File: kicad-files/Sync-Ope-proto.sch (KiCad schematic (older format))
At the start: 59 parts, among them J1 rca, J10 rca, J2 euro_power, J3 mono_jack, J4 mono_jack, J5 mono_jack, J6 rca, J7 AC_POWER, J8 diy_power_header, J9 rca, U1 AD8072, U2 LM1881, U3 L7805, U4 L7905, U5 LT1251, U6 CD4053BE

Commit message: circuit revision 0.3
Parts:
- removed C14: 1nF, symbol Sync-Ope-proto-rescue:C-Device
- removed C3, C4: 100n, Capacitor_THT:C_Disc_D4.3mm_W1.9mm_P5.00mm, symbol Sync-Ope-proto-rescue:C-Sync-Ope-proto-Sync-Ope-proto-rescue
- removed CD4069: delay clamping signal, symbol Sync-Ope-proto-rescue:CD4069
- removed D1: video signal indicator LED, LED_THT:LED_D3.0mm, symbol Sync-Ope-proto-rescue:LED-Device
- removed D2, D3: 1n4148, Diode_THT:D_DO-35_SOD27_P7.62mm_Horizontal, symbol Sync-Ope-proto-rescue:D-Device
- removed R10: 100k, Resistor_THT:R_Axial_DIN0204_L3.6mm_D1.6mm_P7.62mm_Horizontal, symbol Sync-Ope-proto-rescue:R-Device
- removed R14: 10k, Resistor_THT:R_Axial_DIN0204_L3.6mm_D1.6mm_P7.62mm_Horizontal, symbol Sync-Ope-proto-rescue:R-Device
- removed R16: 39k, Resistor_THT:R_Axial_DIN0204_L3.6mm_D1.6mm_P7.62mm_Horizontal, symbol Sync-Ope-proto-rescue:R-Device
- removed R21: 3.3K, symbol Sync-Ope-proto-rescue:R-Device
- removed R3: 220, Resistor_THT:R_Axial_DIN0204_L3.6mm_D1.6mm_P7.62mm_Horizontal, symbol Sync-Ope-proto-rescue:R-Device
- removed R5: 1k, Resistor_THT:R_Axial_DIN0204_L3.6mm_D1.6mm_P7.62mm_Horizontal, symbol Sync-Ope-proto-rescue:R-Sync-Ope-proto-Sync-Ope-proto-rescue
- removed R9: 680k, Resistor_THT:R_Axial_DIN0204_L3.6mm_D1.6mm_P7.62mm_Horizontal, symbol Sync-Ope-proto-rescue:R-Sync-Ope-proto-Sync-Ope-proto-rescue
- removed U2: LM1881, Package_DIP:DIP-8_W7.62mm_LongPads, symbol Sync-Ope-proto-rescue:LM1881-Sync-Ope-proto-Sync-Ope-proto-rescue
- removed U6: CD4053BE, Package_DIP:DIP-16_W7.62mm_LongPads, symbol Sync-Ope-proto-rescue:4053-4xxx
- added C14, C15, C16, C17, C18, C19: 0.1u, Capacitor_THT:C_Disc_D4.3mm_W1.9mm_P5.00mm, symbol Device:C_Small
- added R3: 510, Resistor_THT:R_Axial_DIN0204_L3.6mm_D1.6mm_P7.62mm_Horizontal, symbol Sync-Ope-proto-rescue:R-Sync-Ope-proto-Sync-Ope-proto-rescue
- added R5: 39k, Resistor_THT:R_Axial_DIN0204_L3.6mm_D1.6mm_P7.62mm_Horizontal, symbol Sync-Ope-proto-rescue:R-Device
- C2, C5, C7, C9: value 100n -> 0.1u
- C6, C8: value 330n -> 0.33u
- D7: value schottky -> bat46
- J1, J10, J6, J9: footprint lib_fp:RCJ-024 -> lib_fp:tht_vertical_rca
- J2: value euro_power -> europower
- J3, J4, J5: value mono_jack -> mono_jack_3.5mm
- J7: value AC_POWER -> barrel_jack
- R18: symbol Sync-Ope-proto-rescue:R-Sync-Ope-proto-Sync-Ope-proto-rescue -> Device:R
- RV1: value 10k -> 10k_pot
- U1: footprint Package_DIP:DIP-8_W7.62mm_LongPads -> lib_fp:DIP-SOIC-8
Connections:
- net +5V: now also C14.1, C15.1, C16.1, C17.1, R5.1
- net -5V: now also C18.2, C19.2
- net GND: now also R12.1, C14.2, C15.2, C16.2, C17.2, C18.1, C19.1; no longer J4.TN, R12.2
- net at D6.1 (K), D7.1 (K), U5.1 (IN_1): now also R12.2, R13.1; no longer R12.1, R13.2
- net blanking/return_blank: now reaches J4.T, J9.1 (In)
- net blanking/return_blank: now also R13.2; no longer R13.1
- net at J5.TN: now also R5.2
- net blanking/control_blank: now reaches J5.T
- net ADDED_SYNC renamed blanking/control_pulse
- net DRY_BLANKED_SIGNAL renamed blanking/input_blank
- net VIDEO_TO_SYNC renamed blanking/video_in
- net blanking/video_in: now also R3.2; no longer U1.3 (+)
- new net: R3.1, U1.3 (+)
- no-connect marks 14 -> 12
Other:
- note added: "DRY/WET"
- note removed: "Signal Blanking"
- note removed: "Video Sync Seperator"
- moved on the sheet: C10, C11, C12, C13, C2, C5, C6, C7, C8, C9, D4, D5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

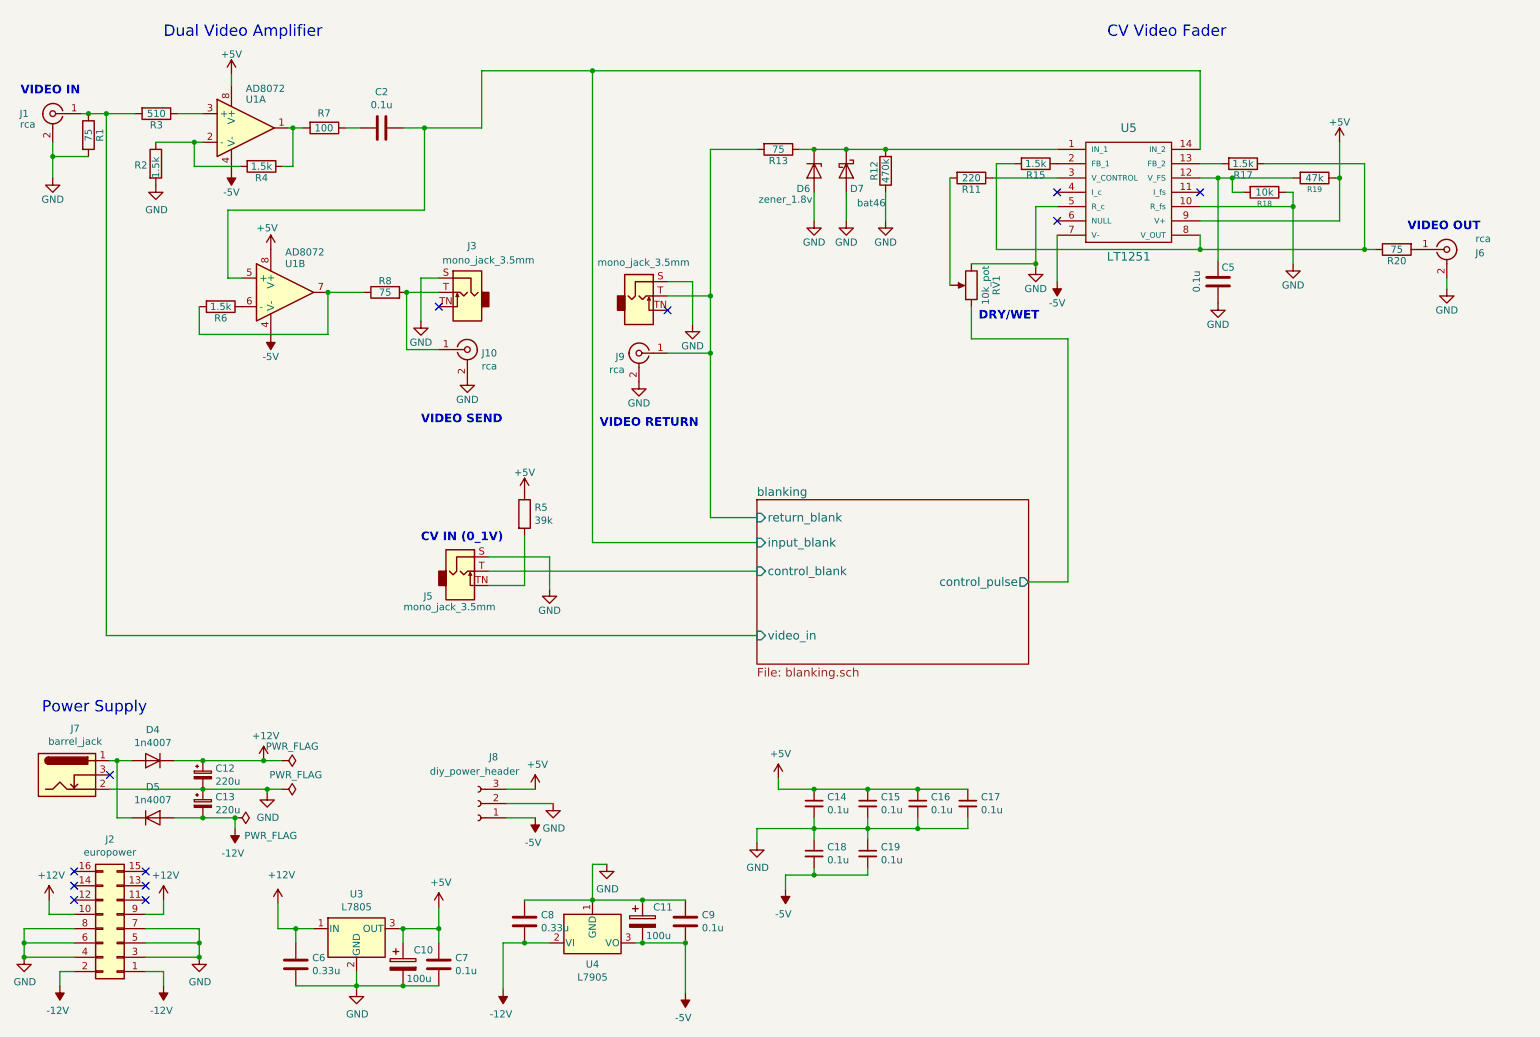
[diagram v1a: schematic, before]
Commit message: working on v0.4.0
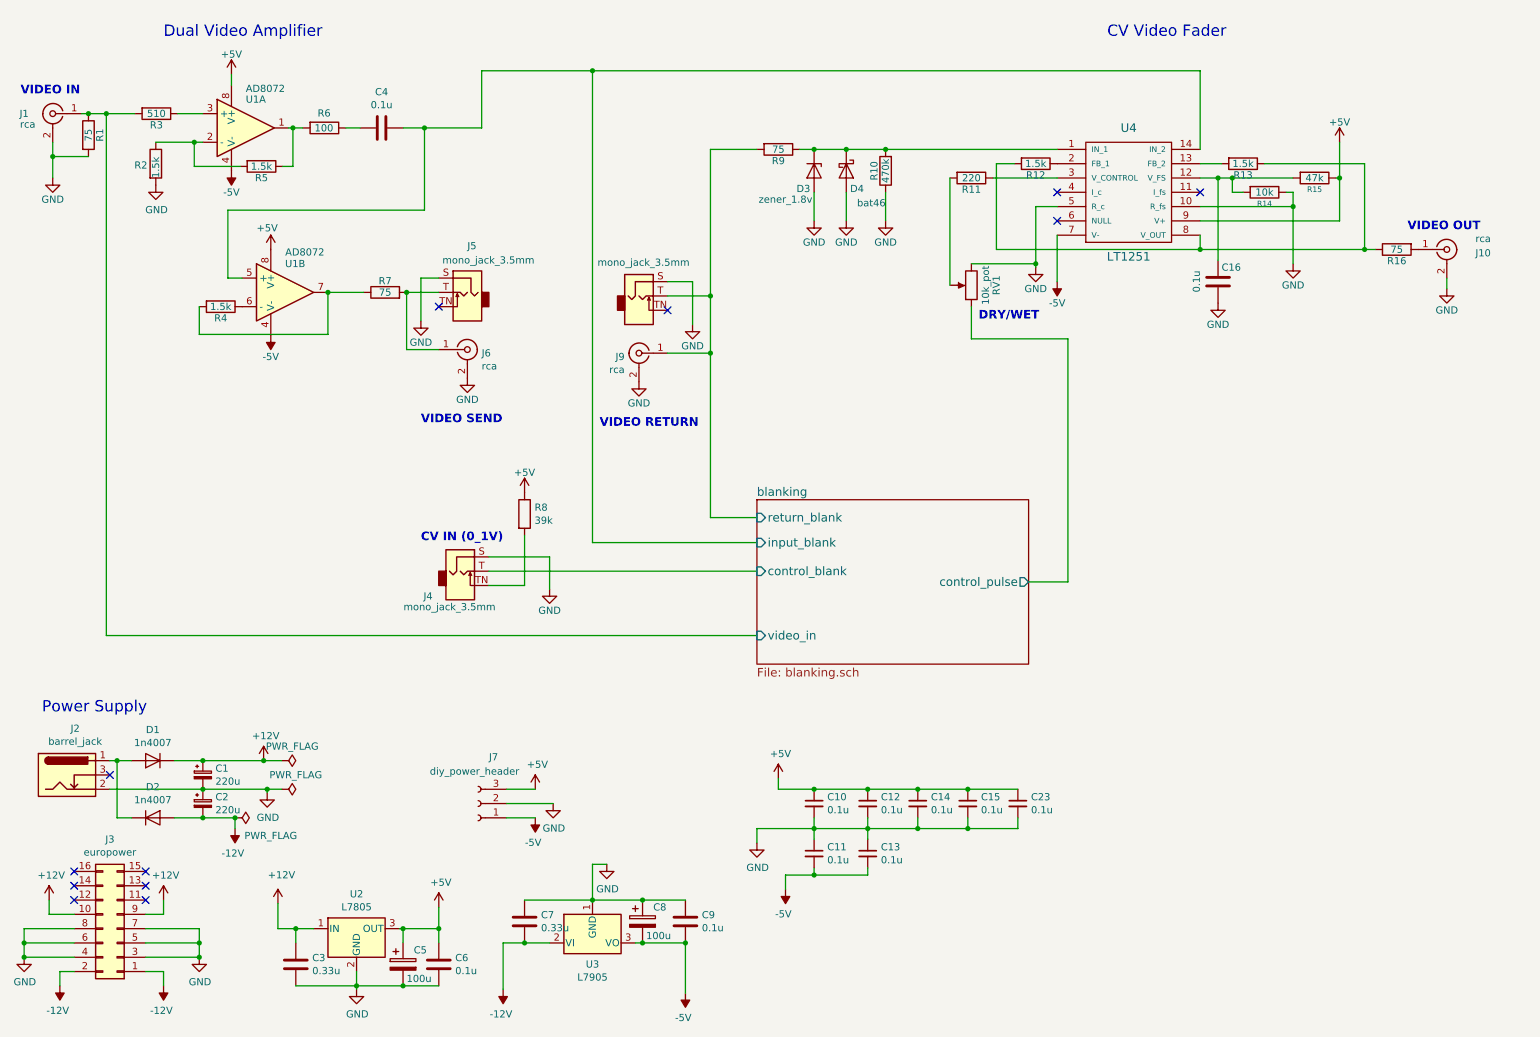
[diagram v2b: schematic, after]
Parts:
- added C23: 0.1u, Capacitor_THT:C_Disc_D4.3mm_W1.9mm_P5.00mm, symbol Device:C_Small
- RV1: footprint Potentiometer_THT:Potentiometer_Alps_RK09K_Single_Vertical -> lib_fp:Potentiometer_Vertical_Large
- U4: renamed from U5; footprint Package_DIP:DIP-14_W7.62mm_Socket_LongPads -> lib_fp:DIP+SOIC_14
- renumbered C12 to C1, C14 to C10, C18 to C11, C15 to C12, C19 to C13, C16 to C14, C17 to C15, C5 to C16, C13 to C2, C6 to C3, C2 to C4, C10 to C5, C7 to C6, C8 to C7, C11 to C8, D4 to D1, D5 to D2, D6 to D3, D7 to D4, J6 to J10, J7 to J2, J2 to J3, J5 to J4, J3 to J5, J10 to J6, J8 to J7, J4 to J8, R12 to R10, R15 to R12, R17 to R13, R18 to R14, R19 to R15, R20 to R16, R6 to R4, R4 to R5, R7 to R6, R8 to R7, R5 to R8, R13 to R9, U3 to U2, U4 to U3
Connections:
- net +5V: now also C23.1
- net GND: now also C23.2
